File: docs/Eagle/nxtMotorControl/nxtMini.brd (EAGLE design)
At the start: 68.3 x 46 mm, 18 parts, among them J11 RJ12, J3 RJ12, J7 Interface

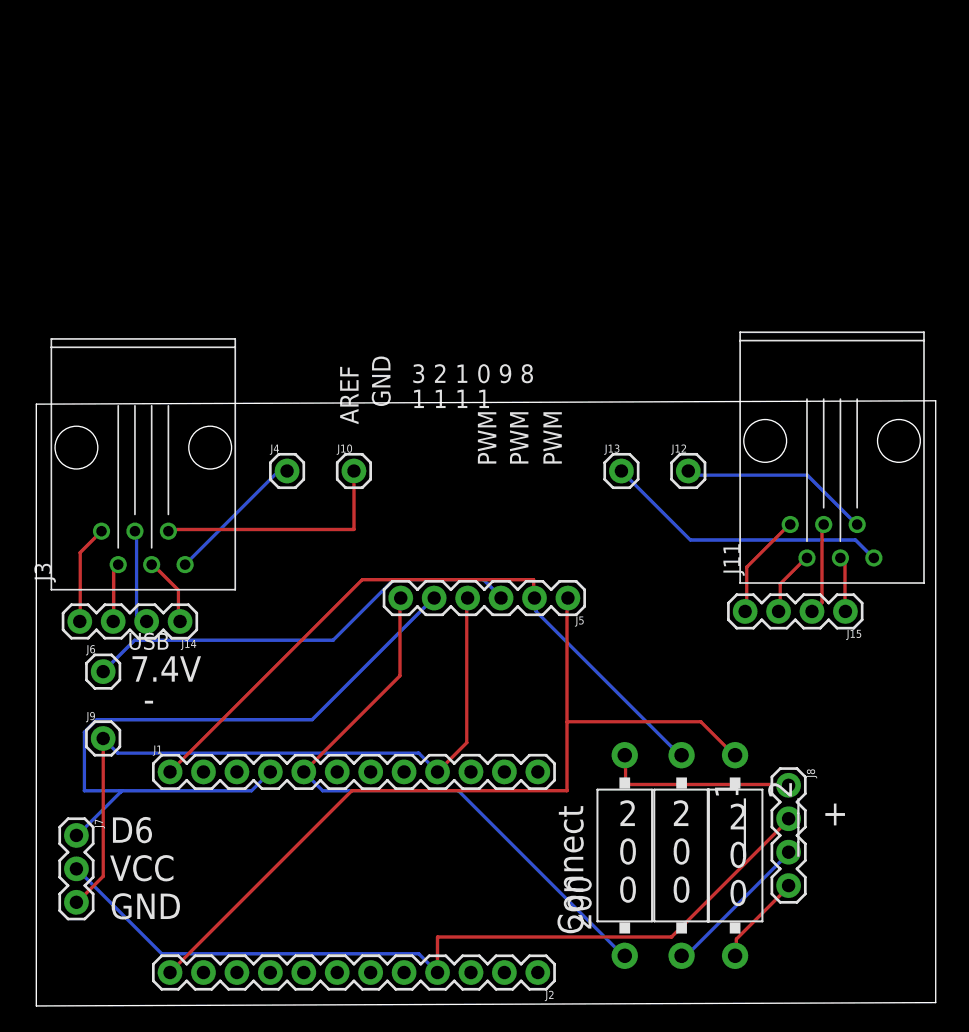
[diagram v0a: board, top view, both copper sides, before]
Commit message: hyo
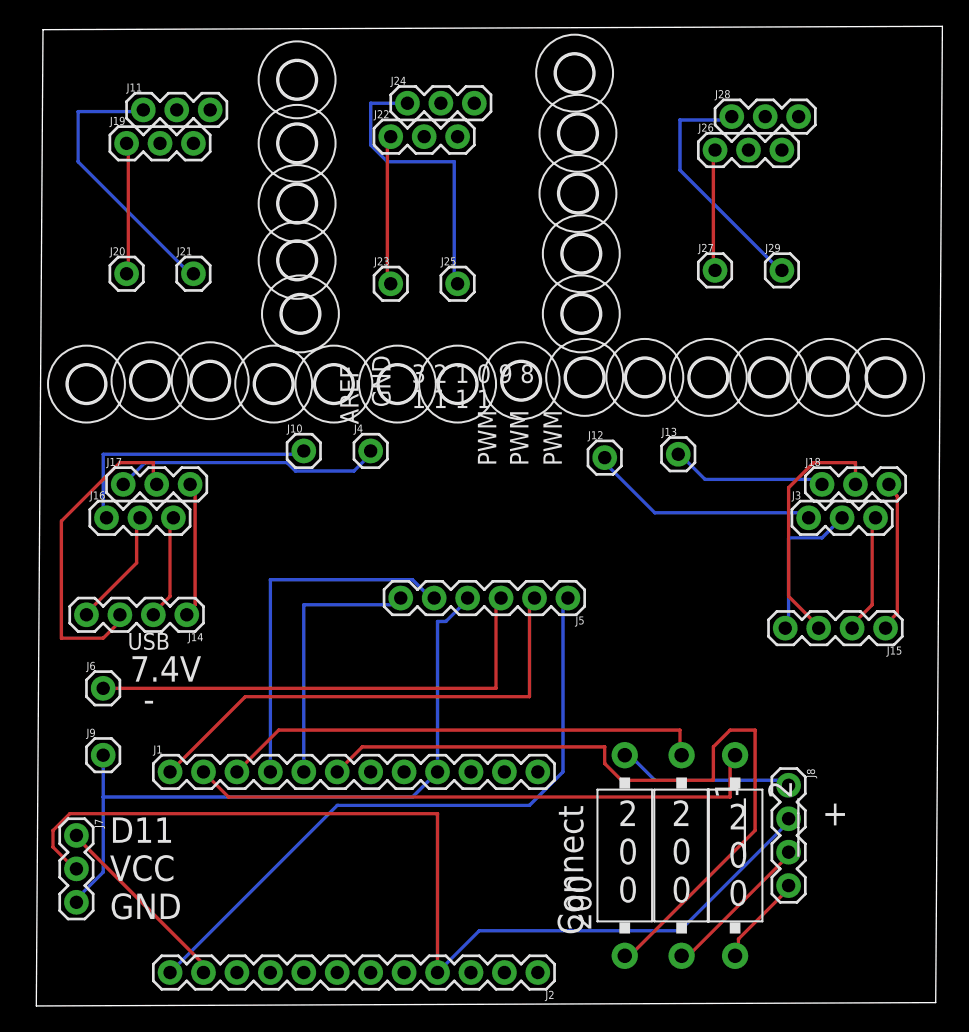
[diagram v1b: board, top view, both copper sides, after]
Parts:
- added J16, J17, J18, J19, J22, J24, J26, J28: 455-1750-1-ND, SparkFun-Connectors:1X03
- added J20, J21, J23, J25, J27, J29: (no value), SparkFun-Connectors:1X01
- added U$1, U$10, U$11, U$12, U$13, U$14, U$15, U$16, U$17, U$18, U$19, U$2, U$20, U$21, U$22, U$23, U$24, U$3, U$4, U$5, U$6, U$7, U$8, U$9: (no value), holes:2,8
- J11, J3: value RJ12 -> 455-1750-1-ND; device con-rj:RJ12 -> SparkFun-Connectors:1X03
- moved J11 58.1 mm to (8.13, 68.1), turned to 0 degrees
- moved J3 50.8 mm to (58.7, 37.1), turned to 0 degrees
- moved J4 6.53 mm to (25.4, 42.2)
- moved J12 6.43 mm to (43.2, 41.7)
- moved J13 4.50 mm to (48.8, 41.9)
- moved J10 4.10 mm to (20.3, 42.2)
- moved J15 3.30 mm to (64.5, 28.7)
- moved J6 1.27 mm to (5.08, 24.1)
- moved J9 1.27 mm to (5.08, 19.1)
- moved J14 0.72 mm to (11.4, 29.7)
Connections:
- new net D4_E: 200.1, J1.6
- new net D7_E: J1.3, ____1.1
- new net D8_E: J1.2, ____2.1
- new net N$16: J19.1, J20.1
- new net N$17: J11.1, J21.1
- new net N$18: J22.1, J23.1
- new net N$19: J24.1, J25.1
- new net N$20: J26.1, J27.1
- new net N$21: J28.1, J29.1
- net D10_E: no longer ____2.1
- net D11_E: now also J7.1
- net D5_E: no longer 200.1
- net D6_E: no longer J7.1
- net D9_E: no longer ____1.1
- net N$1: now also J17.1; no longer J3.1
- net N$10: now also J14.2, J16.3; no longer J14.3, J3.5
- net N$11: now also J14.1, J17.3; no longer J14.4, J3.6
- net N$12: now also J15.4, J3.2; no longer J11.3, J15.1
- net N$13: now also J15.3, J18.2; no longer J11.4, J15.2
- net N$14: now also J15.2, J3.3; no longer J11.5, J15.3
- net N$15: now also J15.1, J18.3; no longer J11.6, J15.4
- net N$2: now also J16.1; no longer J3.2
- net N$6: now also J3.1; no longer J11.2
- net N$7: now also J18.1; no longer J11.1
- net N$8: now also J14.4, J16.2; no longer J14.1, J3.3
- net N$9: now also J14.3, J17.2; no longer J14.2, J3.4
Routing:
- net D4_E: track 0.00 -> 58.9 mm
- net D8_E: track 0.00 -> 44.4 mm
- net D7_E: track 0.00 -> 37.0 mm
- net D6_E: track 54.8 -> 27.6 mm
- net D5_E: track 46.4 -> 20.3 mm
- net N$19: track 0.00 -> 22.2 mm
- net N$17: track 0.00 -> 21.0 mm
- net N$21: track 0.00 -> 18.8 mm
- net N$9: track 7.72 -> 24.9 mm
- net D10_E: track 64.4 -> 49.5 mm
- net D9_E: track 51.8 -> 37.3 mm
- net D11_E: track 0.00 -> 14.4 mm
- net VCC_E: track 63.8 -> 77.2 mm
- net N$13: track 7.04 -> 19.1 mm
- net N$18: track 0.00 -> 11.5 mm
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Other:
- board size 68.3 x 46 mm -> 68.8 x 74.4 mm
- board text added: "D11 VCC GND"
- board text removed: "D6 VCC GND"
